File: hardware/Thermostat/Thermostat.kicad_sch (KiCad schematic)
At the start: 47 parts, among them J1 Barrel_Jack_Switch, J2 Conn_01x02_Pin, J3 AVR-ISP-6, J4 MainConnectorr, K1 G6E, K2 G6E, K3 G6E, K4 G6E, SW1 12MM, SW2 12MM, SW3 12MM, SW4 DIP-1, SW5 SW_Push, SW7 12MM, SW9 12MM, U1 GU112X16G-7003BL, U2 47L04, U4 UA78M05QDCYRQ1, U5 ATmega168P-20A, U8 DS1307Z+, U9 SHT4x, Y1 Crystal, Y3 Crystal

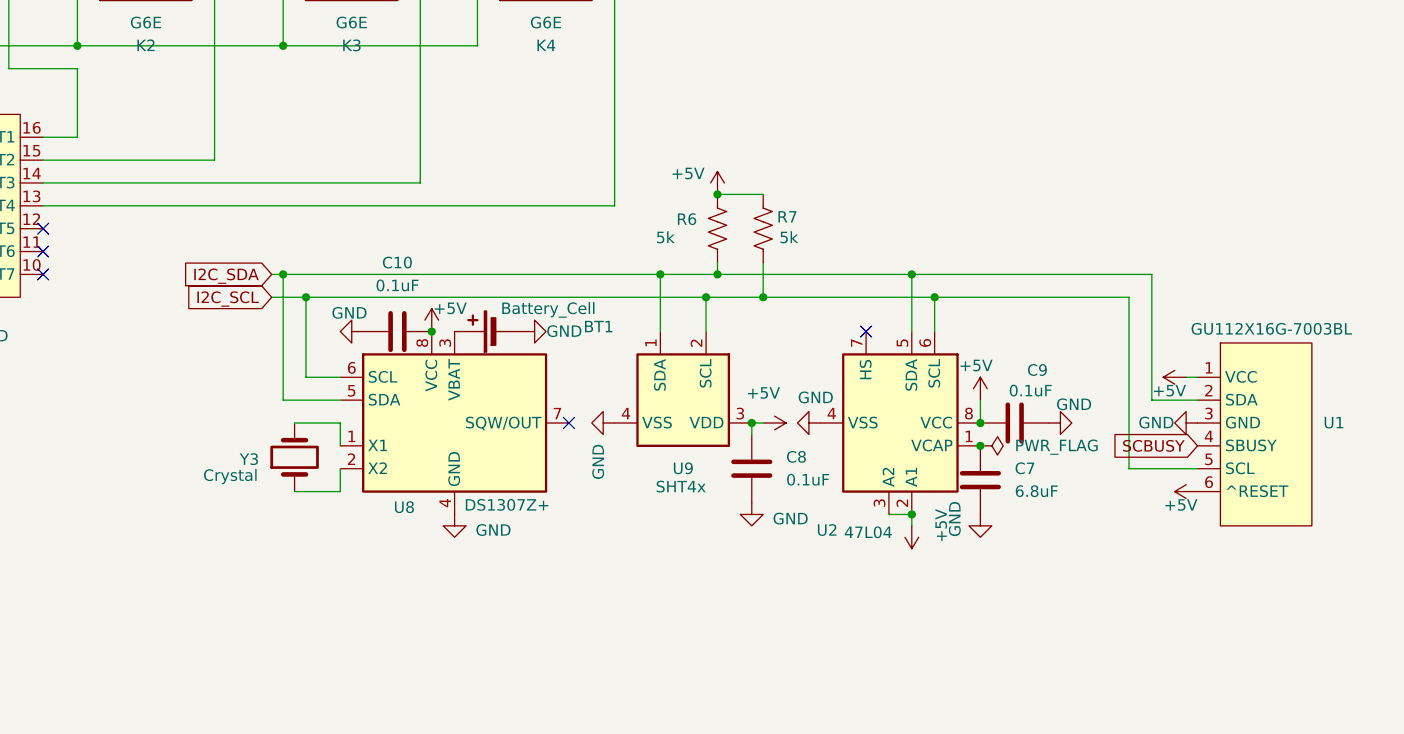
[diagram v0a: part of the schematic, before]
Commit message: Get in battery
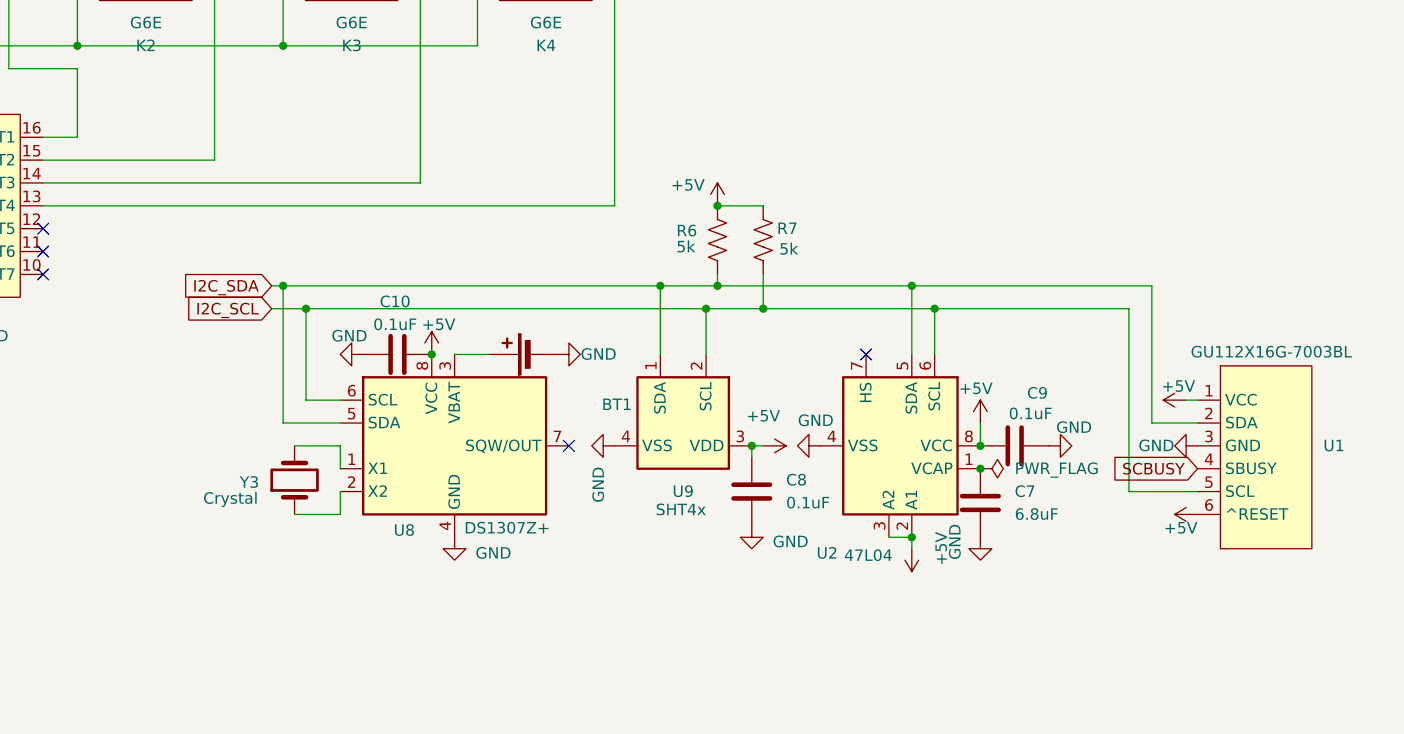
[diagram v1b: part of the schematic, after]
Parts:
- BT1: footprint Battery:BatteryHolder_LINX_BAT-HLD-012-SMT -> Battery:BatteryHolder_Keystone_3000_1x12mm
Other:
- moved on the sheet: BT1, C10, C7, C8, C9, R6, R7, U1, U2, U8, U9, Y3
